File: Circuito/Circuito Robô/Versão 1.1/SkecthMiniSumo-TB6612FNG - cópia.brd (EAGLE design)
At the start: 99 x 75.9 mm, 25 parts, among them IC1 LM317MB, U1 328P, Y1 16MHz

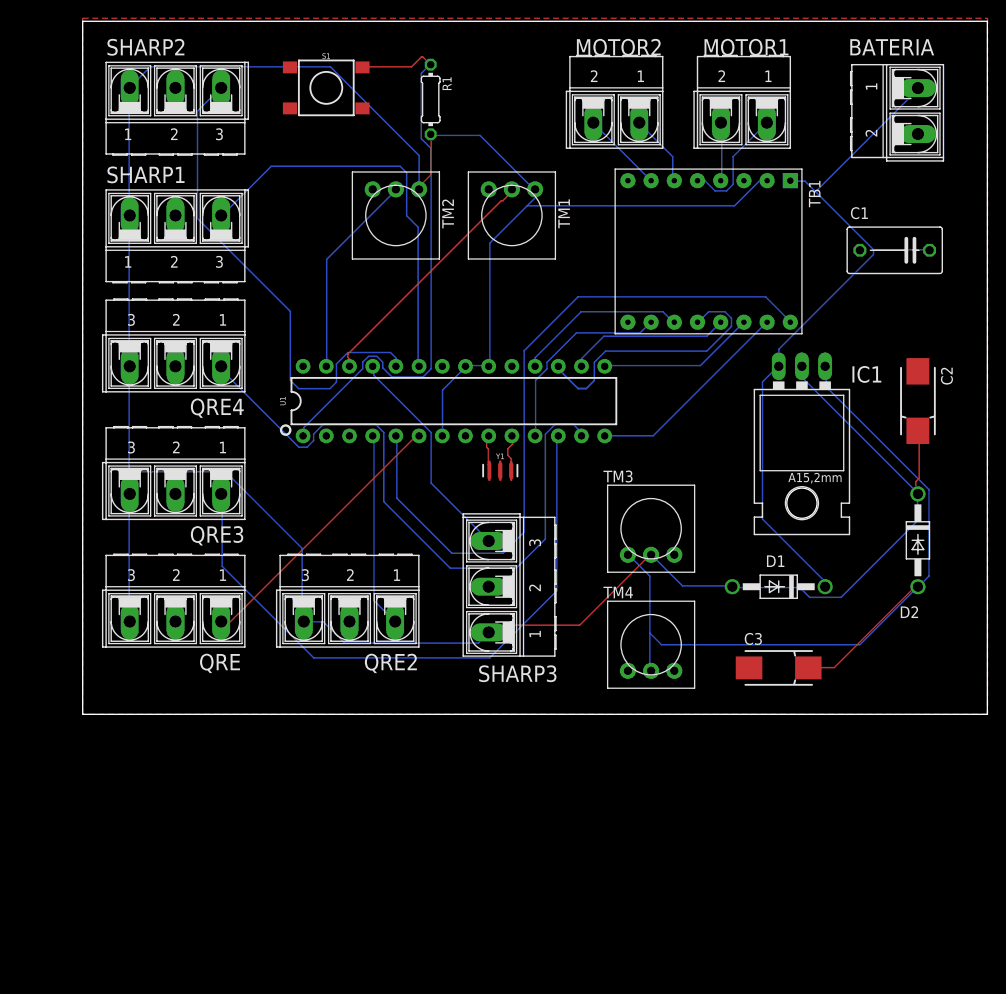
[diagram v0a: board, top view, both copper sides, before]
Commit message: Versão pós Luan
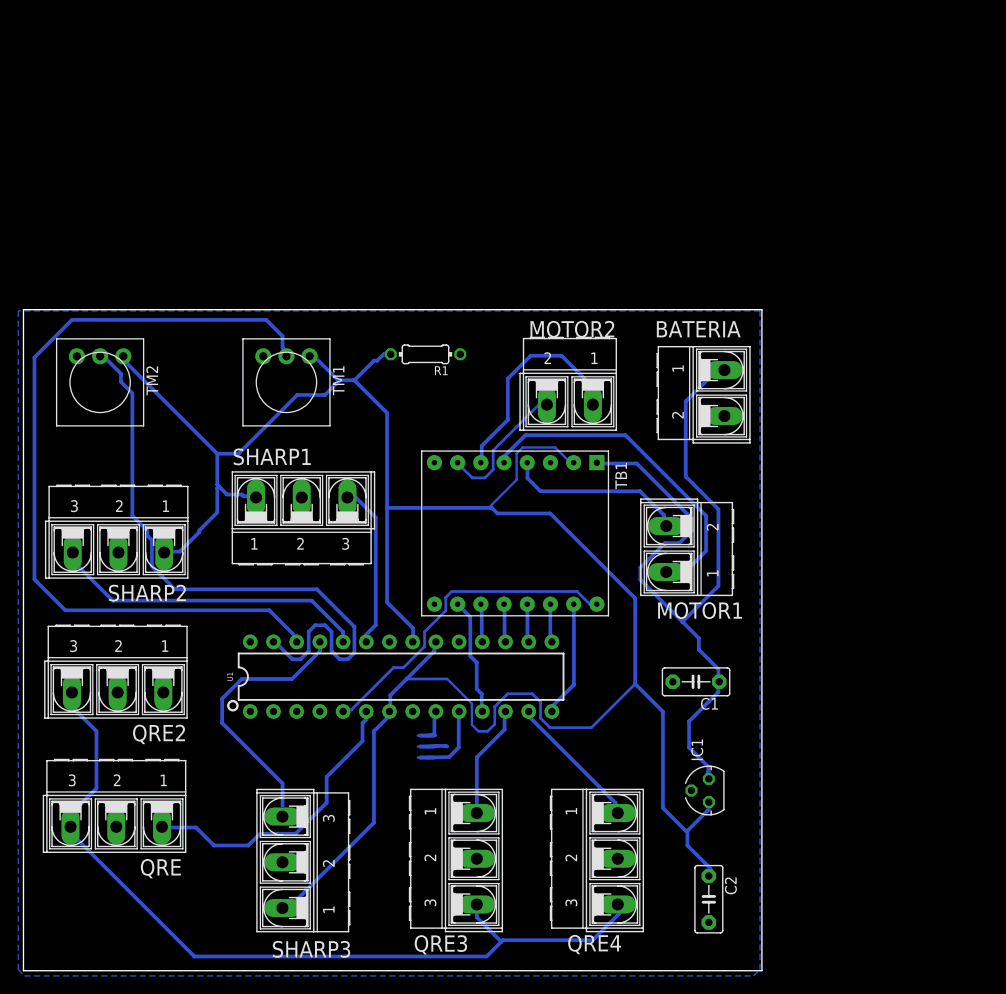
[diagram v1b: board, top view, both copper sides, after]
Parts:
- removed C3: 10uF, resistor:085CS_1AR
- removed D1, D2: 1N4002, diode:DO41-10
- removed S1: MOMENTARY-SWITCH-SPST-SMD-6.2MM-TALL, SparkFun-Switches:TACTILE_SWITCH_SMD_6.2MM_TALL
- removed TM3, TM4: (no value), adafruit:TRIM-3386
- C1: value 0.1uF -> (none); device rcl:C075-052X106 -> capacitor-wima:C5B3
- C2: value 1uF -> (none); device resistor:085CS_1AR -> capacitor-wima:C5B3
- IC1: value LM317MB -> (none); device v-reg:TO220L1 -> v-reg:78LXX
- moved QRE4 72.5 mm to (64.9, 12.1), turned to 270 degrees
- moved C2 59.1 mm to (74.9, 7.70)
- moved C1 52.0 mm to (73.5, 31.5)
- moved QRE3 51.8 mm to (49.5, 12.1), turned to 270 degrees
- moved SHARP2 51.3 mm to (10.3, 45.6), turned to 180 degrees
- moved MOTOR1 47.4 mm to (70.2, 46.0), turned to 90 degrees
- moved IC1 43.8 mm to (74.9, 19.6), turned to 90 degrees
- moved SHARP3 37.7 mm to (28.2, 11.7)
- moved BATERIA 37.4 mm to (76.6, 63.1)
- moved TB1 37.4 mm to (56.3, 47.9)
- moved TM2 37.2 mm to (8.26, 64.3)
- moved SHARP1 33.8 mm to (30.3, 51.7)
- moved MOTOR2 31.3 mm to (59.7, 61.8)
- moved Y1 31.2 mm to (44.0, 24.4), flipped to the bottom, turned to 270 degrees
- moved U1 30.7 mm to (41.2, 32.1)
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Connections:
- removed net N$13: C3.+, D2.A, IC1.1, TM3.1, TM4.2
- removed net N$3: R1.1, S1.B2, U1.1
- new net N$32: QRE.3, QRE2.3, QRE3.3, QRE4.3
- net GND: now also C2.2, IC1.GND, R1.1, U1.1; no longer C2.-, C3.-, S1.A2, TM4.1
- net VIN: now also IC1.IN; no longer D1.C, IC1.3
- net VO: now also C2.1, IC1.OUT; no longer C2.+, D1.A, D2.C, IC1.2, QRE.3, QRE2.3, QRE3.3, QRE4.3, TM3.2
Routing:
- net N$32: track 0.00 -> 91.5 mm
- net N$13: track 91.4 -> 0.00 mm
- net VO: track 318.3 -> 249.2 mm
- net N$3: track 62.7 -> 0.00 mm
- net N$25: track 27.0 -> 88.1 mm
- net N$19: track 68.9 -> 12.5 mm
- net N$18: track 69.7 -> 15.2 mm
- net N$23: track 22.5 -> 68.8 mm
- net N$10: track 76.9 -> 35.6 mm
- net N$14: track 44.6 -> 18.1 mm
- net N$12: track 29.5 -> 4.20 mm
- net N$7: track 12.9 -> 36.6 mm
- net N$17: track 21.3 -> 0.00 mm
- net N$15: track 53.2 -> 34.8 mm
- net N$8: track 7.94 -> 24.1 mm
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- added copper zone on layer 16, net GND
- removed copper zone on layer 1, net GND
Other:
- board size 99 x 75.9 mm -> 80.8 x 72.4 mm

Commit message: Placa pseudo pronta
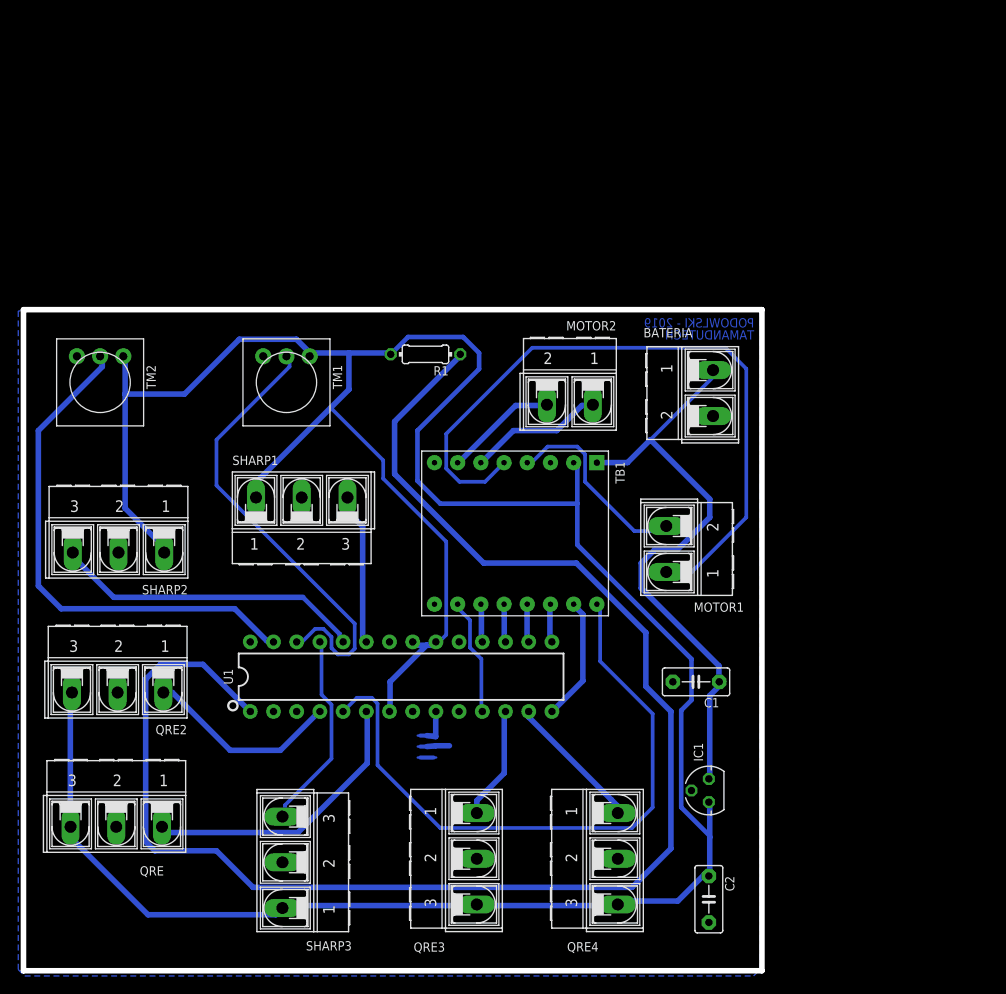
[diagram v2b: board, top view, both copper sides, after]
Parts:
- moved BATERIA 1.25 mm to (75.4, 63.1)
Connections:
- removed net N$32: QRE.3, QRE2.3, QRE3.3, QRE4.3
- new net N$3: R1.1, U1.1
- net GND: no longer R1.1, U1.1
- net VO: now also QRE.3, QRE2.3, QRE3.3, QRE4.3
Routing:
- net N$3: track 0.00 -> 168.9 mm
- net N$32: track 91.5 -> 0.00 mm
- net VO: track 249.2 -> 314.8 mm
- net N$7: track 36.6 -> 76.8 mm
- net N$25: track 88.1 -> 50.9 mm
- net N$10: track 35.6 -> 70.1 mm
- net N$17: track 0.00 -> 21.5 mm
- net VIN: track 83.4 -> 66.4 mm
- net N$23: track 68.8 -> 56.4 mm
- net N$8: track 24.1 -> 14.9 mm
- net N$2: track 7.89 -> 0.00 mm
- net N$16: track 29.5 -> 21.9 mm
- net N$9: track 15.2 -> 12.4 mm
- net N$6: track 19.5 -> 21.7 mm
- net N$14: track 18.1 -> 16.8 mm
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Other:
- board text added: "PODOWLSKI - 2019"
- board text added: "TAMANDUTECH"
